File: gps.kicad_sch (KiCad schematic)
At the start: 10 parts, among them J3 50R SMA_Conn, U6 MAX-M10S

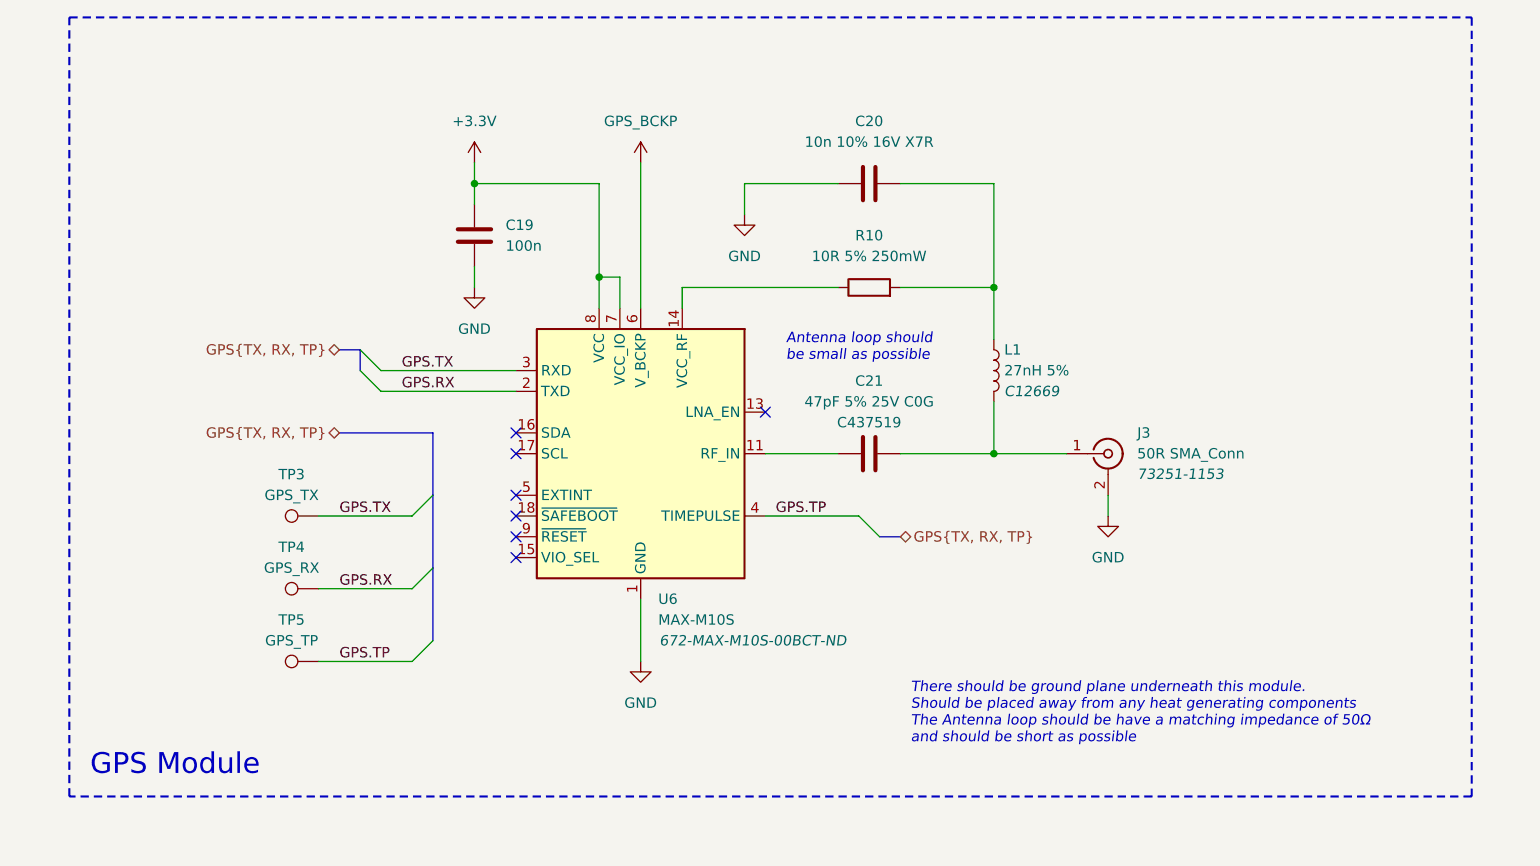
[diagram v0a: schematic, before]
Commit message: Display Driver Completion
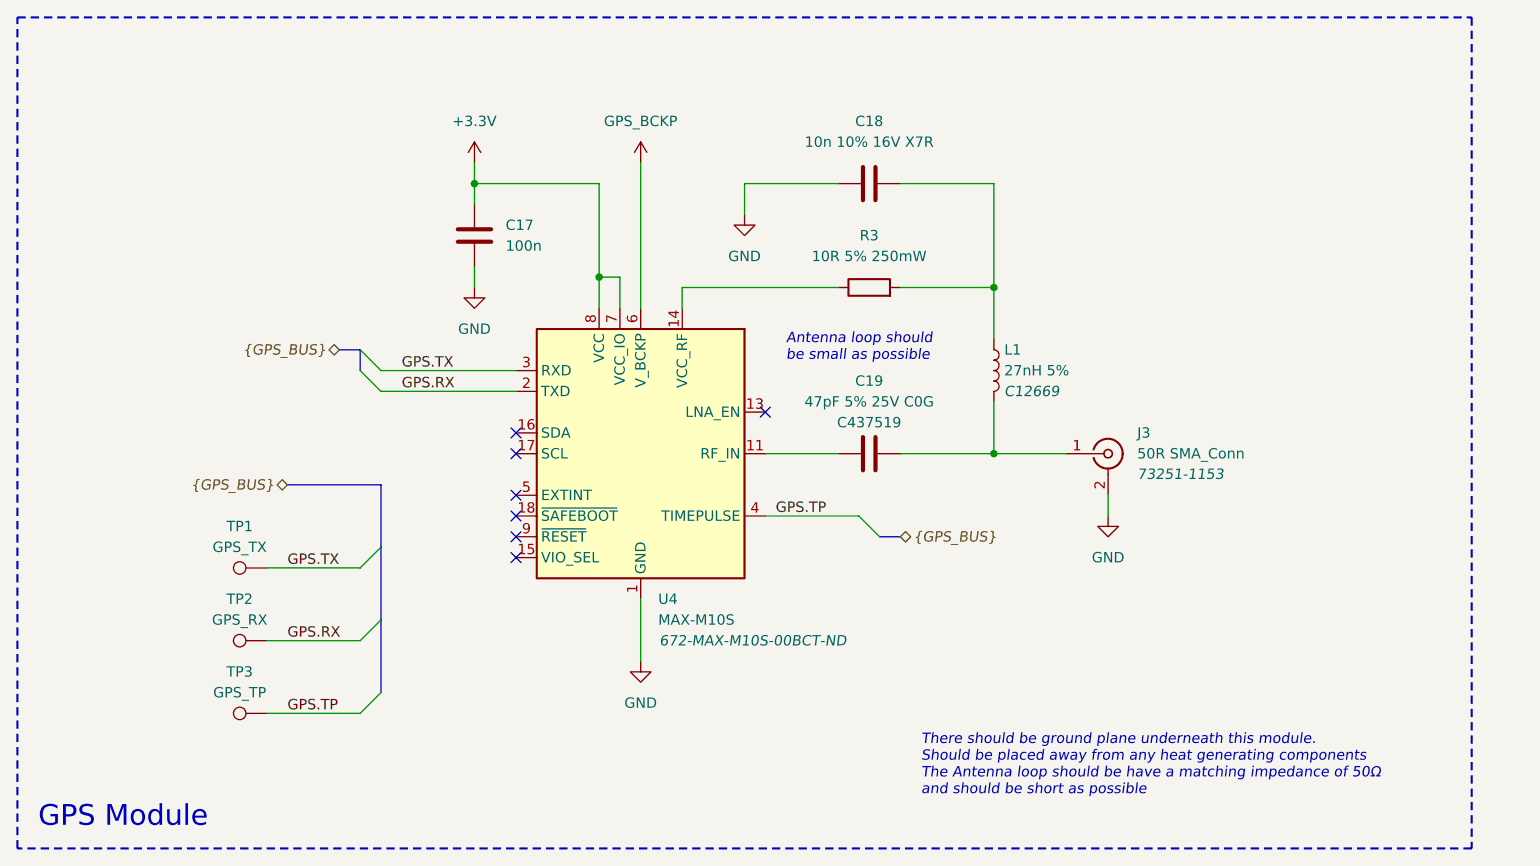
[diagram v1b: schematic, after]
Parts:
- C19: renamed from C21; footprint (none) -> Capacitor_SMD:C_0402_1005Metric
- renumbered C19 to C17, C20 to C18, R10 to R3, TP3 to TP1, TP4 to TP2, TP5 to TP3, U6 to U4
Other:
- moved on the sheet: TP1, TP2, TP3
